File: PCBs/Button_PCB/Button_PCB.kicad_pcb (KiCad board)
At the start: 2 copper layers, 42.5 x 26.8 mm, 4 parts, among them J1 Conn_01x05_Male, J2 RIGHT_BUTTON, J3 MIDDLE_BUTTON, J4 LEFT_BUTTON

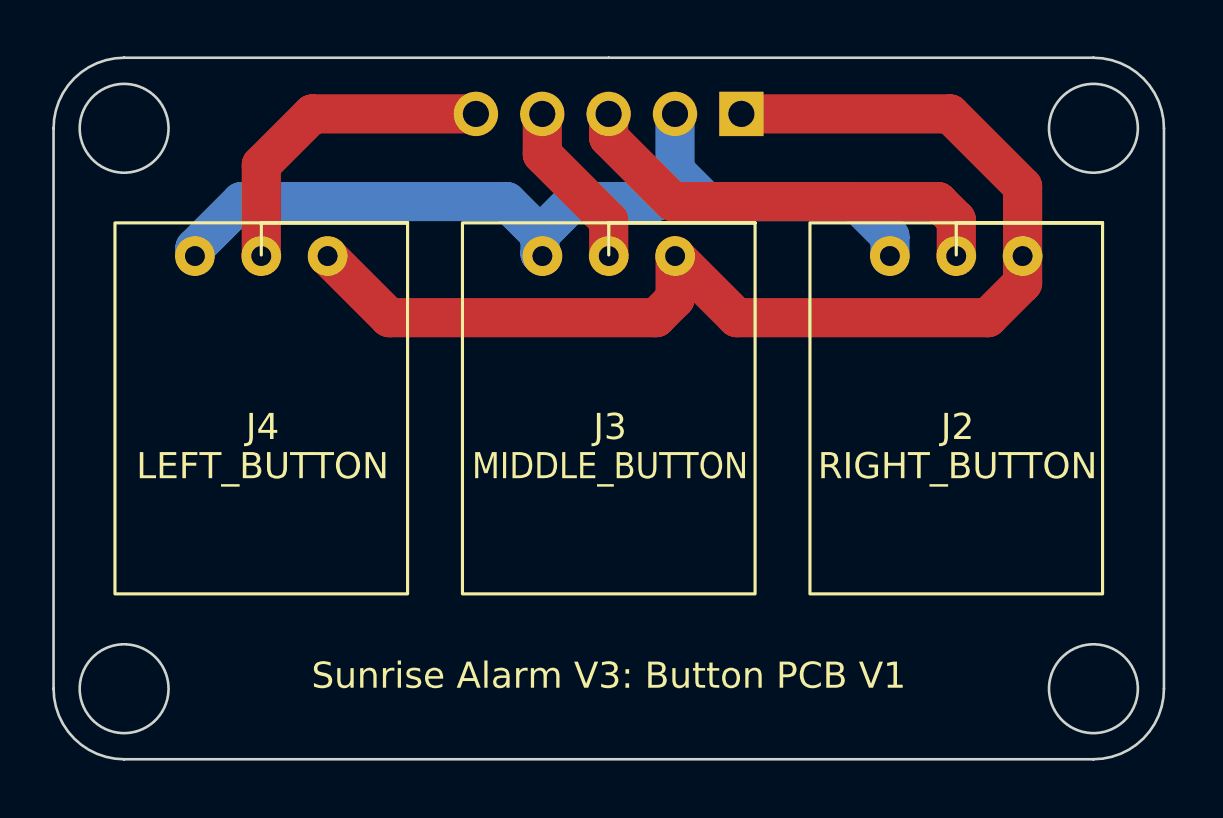
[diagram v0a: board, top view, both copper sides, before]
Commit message: V3.4.3-alpha Generated PCB Gerber Files
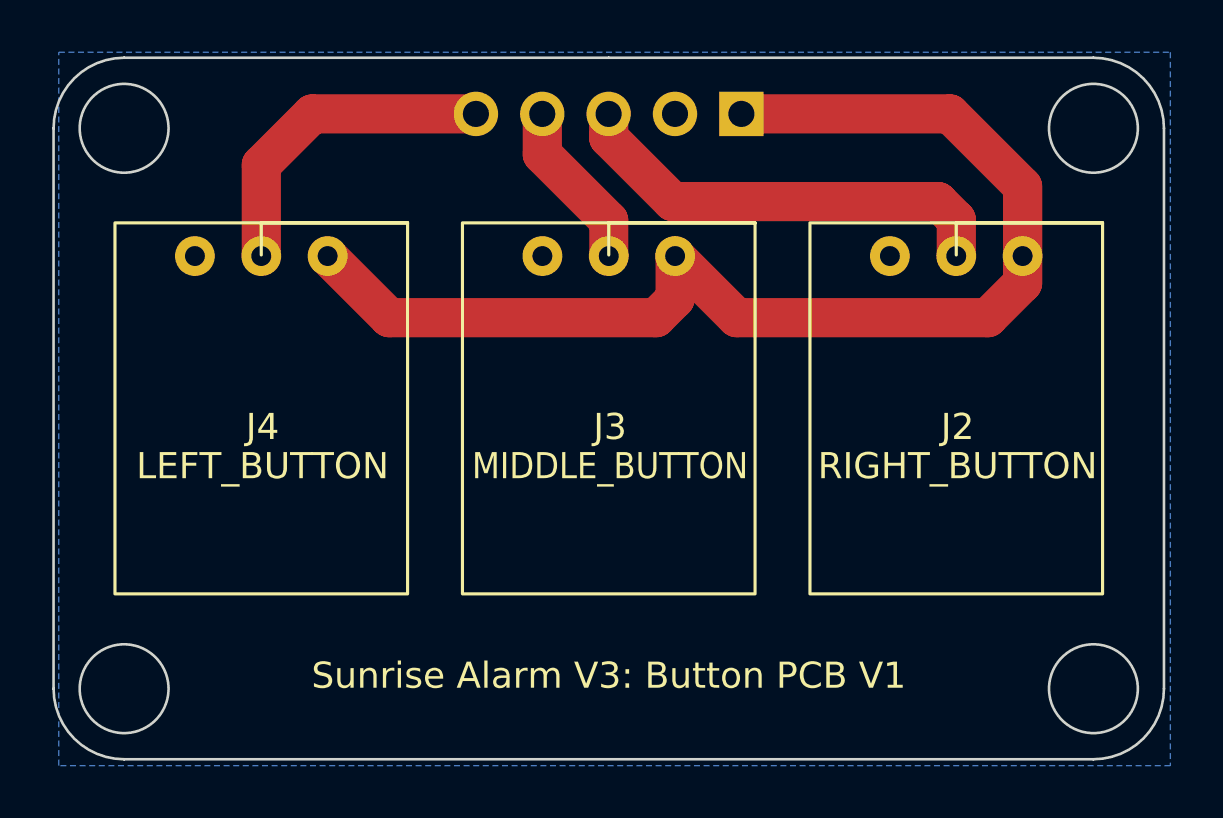
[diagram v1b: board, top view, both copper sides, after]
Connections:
- net Net-(J1-Pad1) renamed VCC
- net Net-(J1-Pad2) renamed GND
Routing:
- net GND: track 34.3 -> 0.00 mm
- added copper zone on B.Cu, net GND
